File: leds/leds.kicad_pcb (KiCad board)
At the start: 4 copper layers, 68.8 x 135.2 mm, 96 parts, among them CN1 39302030, CN2 39288020, CN3 39288020, CN4 39288020, CN5 39302030, CN6 39288020, CN7 39288020, CN701 BM04B-SRSS-TB(LF)(SN), CN8 39288020, J202 Conn_01x06, J301 Conn_01x05_Pin, Q701 BSS138, Q702 BSS138, SW201 KEY-SMD_B3U-1000PM, SW202 KEY-SMD_B3U-1000PM, U1 SN74AHCT125PWR, U2 BTS70021EPPXUMA1, U201 ESP32-S3-WROOM-1, U3 BTS70021EPPXUMA1, U301 TPD6S300A, U302 TPS25730D, U401 TPS54202DDC, U402 CYA1040-15UH, U701 TPS73733DCQ_C5220270

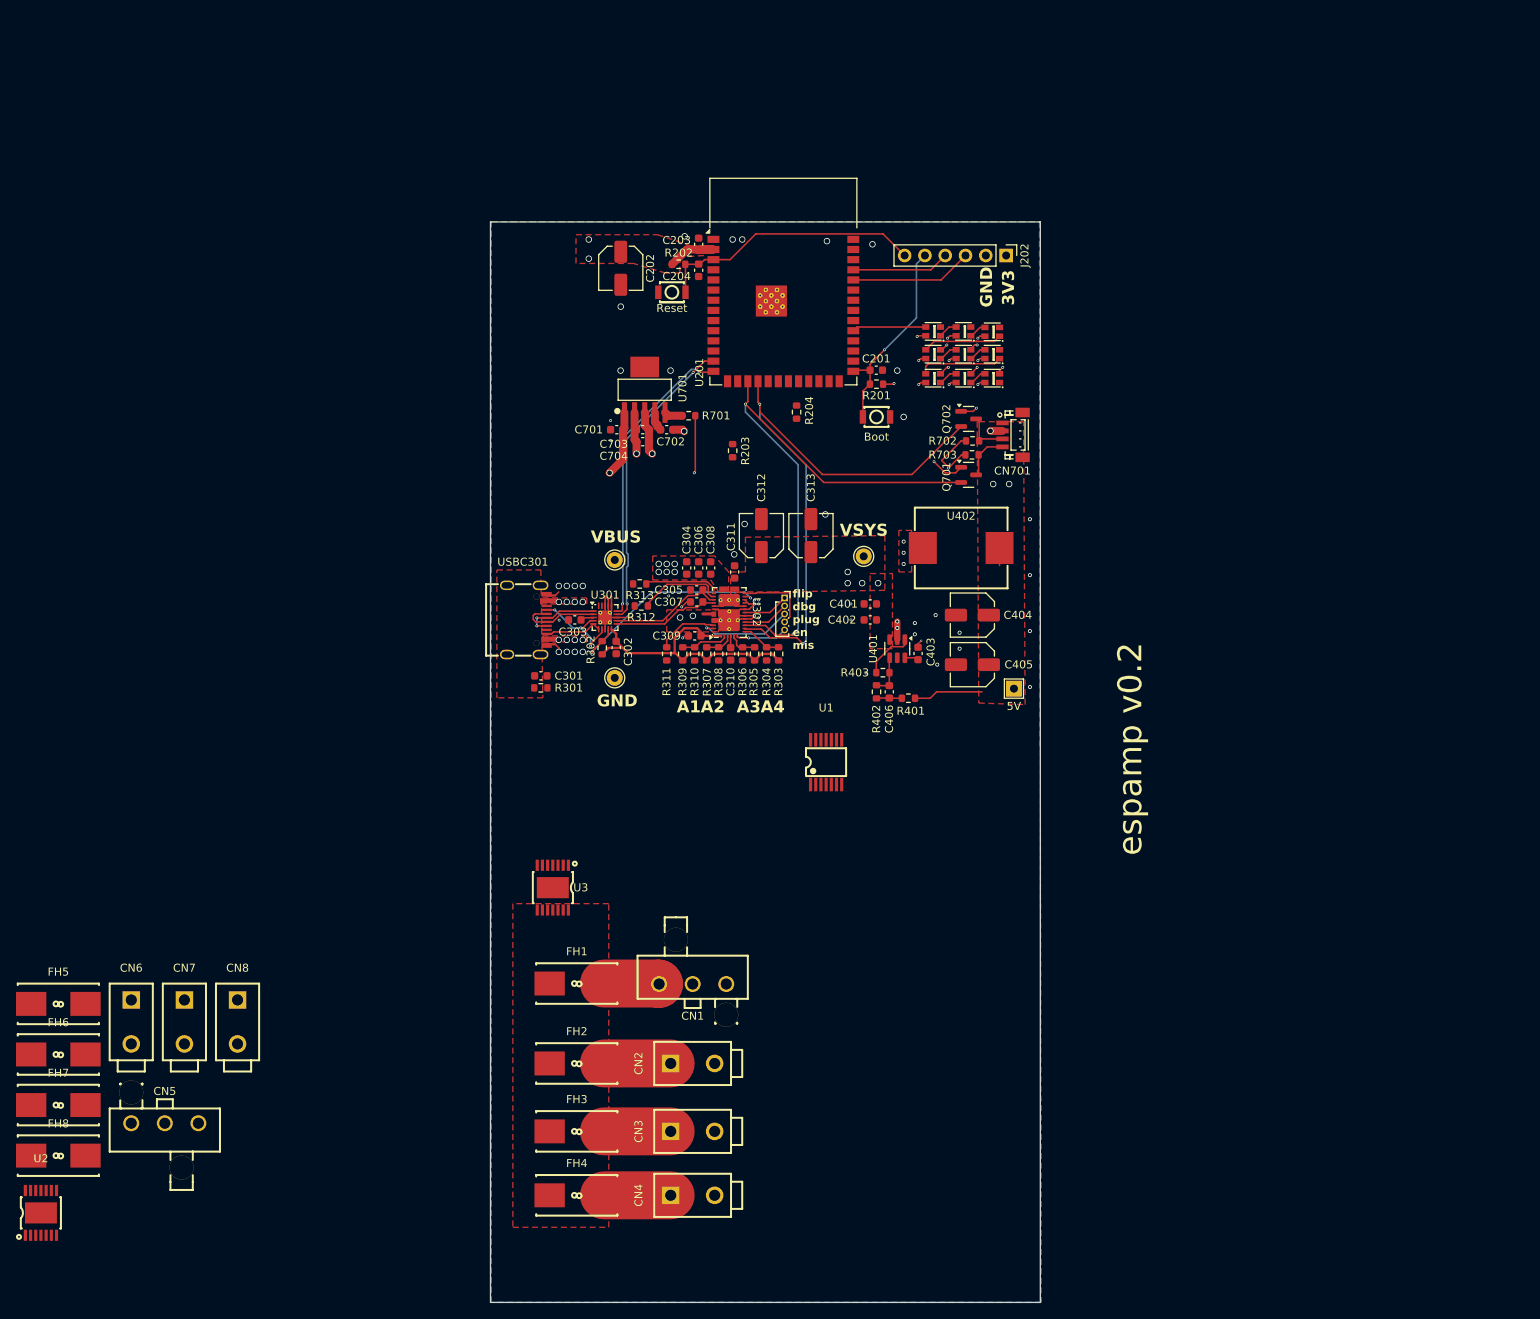
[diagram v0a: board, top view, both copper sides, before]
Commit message: first draft
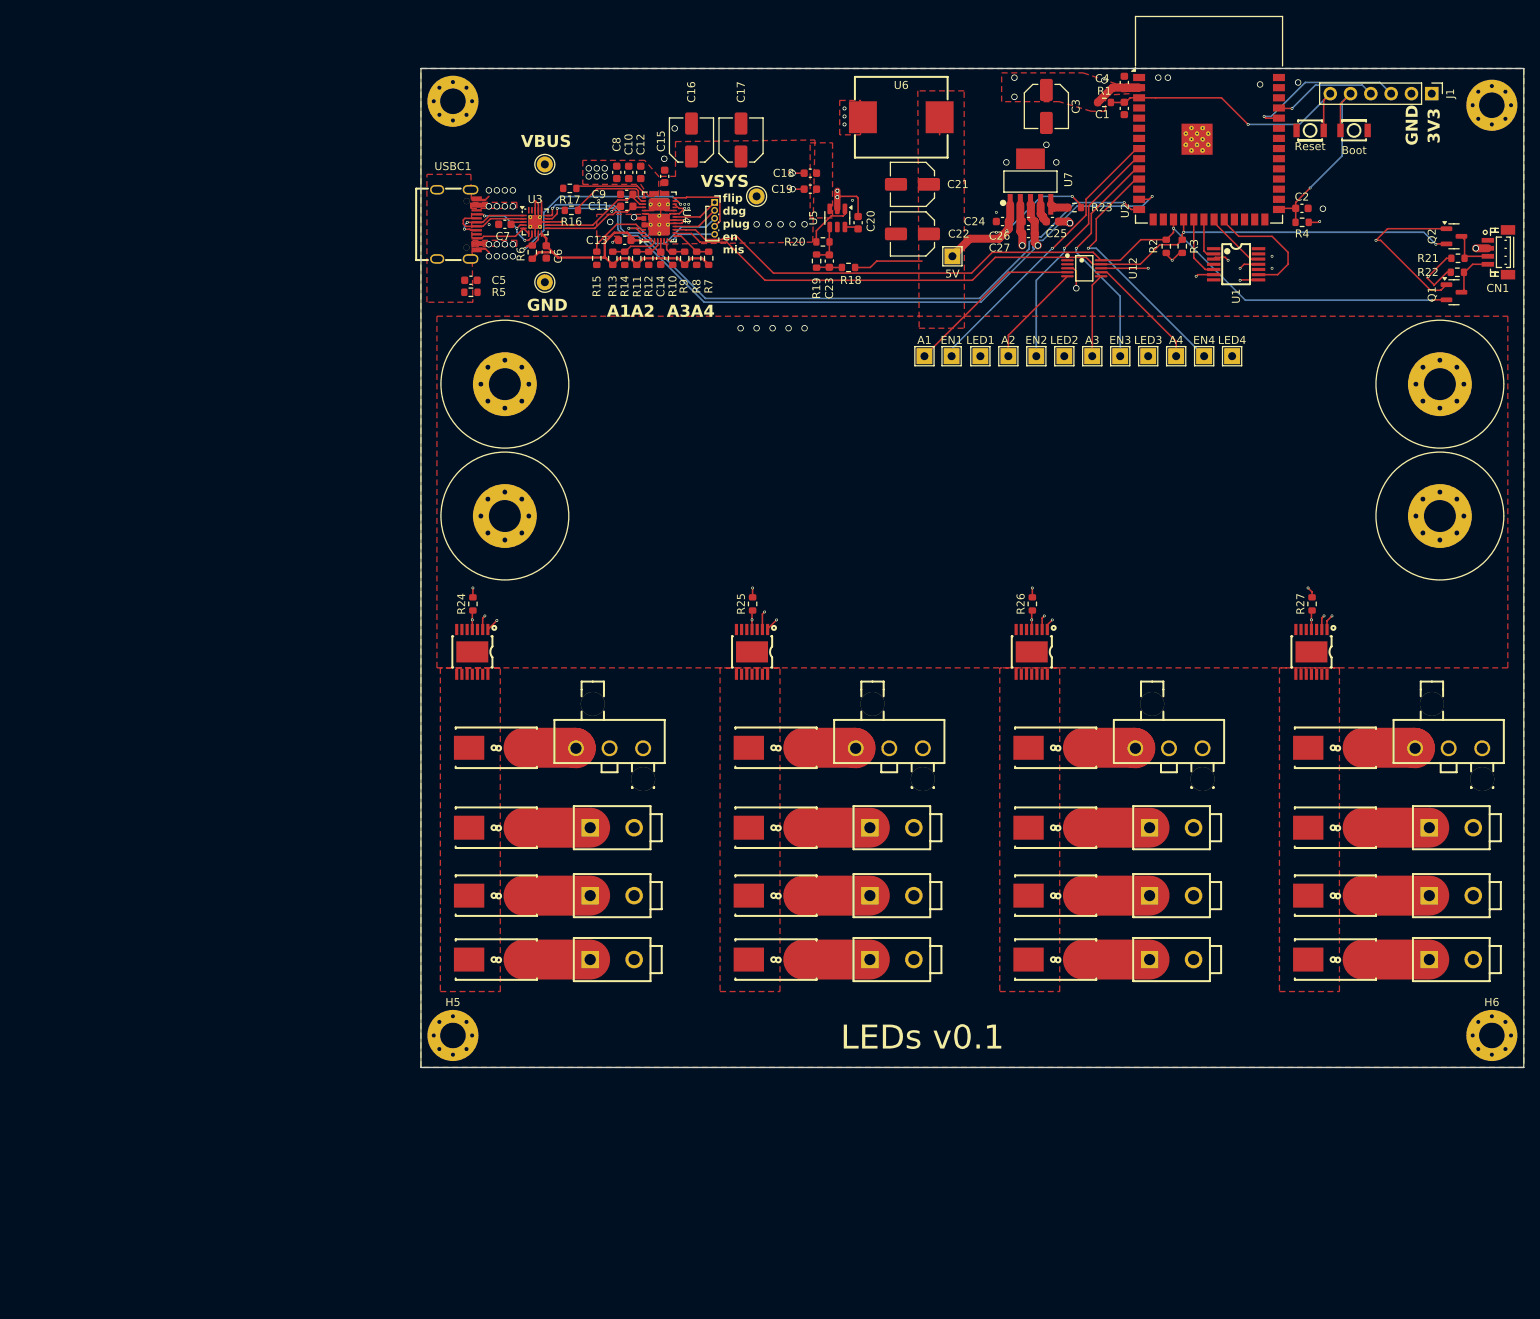
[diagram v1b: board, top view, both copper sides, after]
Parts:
- removed the CN5 at (-20.1, 157.0)
- removed LED201, LED202, LED203, LED204, LED205, LED206, LED207, LED208, LED209: WS2812B-2020, easyeda2kicad:LED-SMD_4P-L2.0-W2.0-TL_WS2812B-2020
- removed the U2 at (-35.5, 168.2)
- added CN10: 39302030, easyeda2kicad:CONN-TH_3P-P4.20_39302030, F.Cu at (105.6, 110.1)
- added CN11: 39288020, easyeda2kicad:CONN-TH_39288020, F.Cu at (105.9, 120.0)
- added CN12: 39288020, easyeda2kicad:CONN-TH_39288020, F.Cu at (105.9, 128.5)
- added CN13: 39288020, easyeda2kicad:CONN-TH_39288020, F.Cu at (105.9, 136.5)
- added CN14: 39302030, easyeda2kicad:CONN-TH_3P-P4.20_39302030, F.Cu at (140.6, 110.1)
- added CN15: 39288020, easyeda2kicad:CONN-TH_39288020, F.Cu at (140.9, 120.0)
- added CN16: 39288020, easyeda2kicad:CONN-TH_39288020, F.Cu at (140.9, 128.5)
- added CN17: 39288020, easyeda2kicad:CONN-TH_39288020, F.Cu at (140.9, 136.5)
- added CN9: 39288020, easyeda2kicad:CONN-TH_39288020, F.Cu at (70.9, 136.5)
- added FH10: 01550900M, easyeda2kicad:FUSE-SMD_L9.8-W5.0_01550900M, F.Cu at (91.4, 120.0)
- added FH11: 01550900M, easyeda2kicad:FUSE-SMD_L9.8-W5.0_01550900M, F.Cu at (91.4, 128.5)
- added FH12: 01550900M, easyeda2kicad:FUSE-SMD_L9.8-W5.0_01550900M, F.Cu at (91.4, 136.5)
- added FH13: 01550900M, easyeda2kicad:FUSE-SMD_L9.8-W5.0_01550900M, F.Cu at (126.4, 110.0)
- added FH14: 01550900M, easyeda2kicad:FUSE-SMD_L9.8-W5.0_01550900M, F.Cu at (126.4, 120.0)
- added FH15: 01550900M, easyeda2kicad:FUSE-SMD_L9.8-W5.0_01550900M, F.Cu at (126.4, 128.5)
- added FH16: 01550900M, easyeda2kicad:FUSE-SMD_L9.8-W5.0_01550900M, F.Cu at (126.4, 136.5)
- added FH9: 01550900M, easyeda2kicad:FUSE-SMD_L9.8-W5.0_01550900M, F.Cu at (91.4, 110.0)
- added H1: MountingHole_Pad, MountingHole:MountingHole_4mm_Pad_Via, F.Cu at (22.5, 81.0)
- added H2: MountingHole_Pad, MountingHole:MountingHole_4mm_Pad_Via, F.Cu at (139.5, 64.5)
- added H3: MountingHole_Pad, MountingHole:MountingHole_4mm_Pad_Via, F.Cu at (139.5, 81.0)
- added H4: MountingHole_Pad, MountingHole:MountingHole_4mm_Pad_Via, F.Cu at (22.5, 64.5)
- added H5: MountingHole_Pad, MountingHole:MountingHole_3.2mm_M3_Pad_Via, F.Cu at (16.0, 146.0)
- added H6: MountingHole_Pad, MountingHole:MountingHole_3.2mm_M3_Pad_Via, F.Cu at (146.0, 146.0)
- added H7: MountingHole_Pad, MountingHole:MountingHole_3.2mm_M3_Pad_Via, F.Cu at (16.0, 29.1)
- added H8: MountingHole_Pad, MountingHole:MountingHole_3.2mm_M3_Pad_Via, F.Cu at (146.0, 29.6)
- added R24: 820, Resistor_SMD:R_0603_1608Metric, F.Cu at (18.5, 92.0)
- added R25: 820, Resistor_SMD:R_0603_1608Metric, F.Cu at (53.5, 92.0)
- added R26: 820, Resistor_SMD:R_0603_1608Metric, F.Cu at (88.5, 92.0)
- added R27: 820, Resistor_SMD:R_0603_1608Metric, F.Cu at (123.5, 92.0)
- added TP10: LabeledTestPoint, easyeda2kicad:LabeledTestPoint, F.Cu at (89.0, 61.0)
- added TP11: LabeledTestPoint, easyeda2kicad:LabeledTestPoint, F.Cu at (99.5, 61.0)
- added TP12: LabeledTestPoint, easyeda2kicad:LabeledTestPoint, F.Cu at (110.0, 61.0)
- added TP13: LabeledTestPoint, easyeda2kicad:LabeledTestPoint, F.Cu at (75.0, 61.0)
- added TP14: LabeledTestPoint, easyeda2kicad:LabeledTestPoint, F.Cu at (85.5, 61.0)
- added TP15: LabeledTestPoint, easyeda2kicad:LabeledTestPoint, F.Cu at (96.0, 61.0)
- added TP16: LabeledTestPoint, easyeda2kicad:LabeledTestPoint, F.Cu at (106.5, 61.0)
- added TP5: LabeledTestPoint, easyeda2kicad:LabeledTestPoint, F.Cu at (82.0, 61.0)
- added TP6: LabeledTestPoint, easyeda2kicad:LabeledTestPoint, F.Cu at (92.5, 61.0)
- added TP7: LabeledTestPoint, easyeda2kicad:LabeledTestPoint, F.Cu at (103.0, 61.0)
- added TP8: LabeledTestPoint, easyeda2kicad:LabeledTestPoint, F.Cu at (113.5, 61.0)
- added TP9: LabeledTestPoint, easyeda2kicad:LabeledTestPoint, F.Cu at (78.4, 61.0)
- added U10: BTS70021EPPXUMA1, easyeda2kicad:PG-TSDSO-14_L4.9-W3.9-P0.65-LS6.0-BL-EP, F.Cu at (88.4, 98.0)
- added U11: BTS70021EPPXUMA1, easyeda2kicad:PG-TSDSO-14_L4.9-W3.9-P0.65-LS6.0-BL-EP, F.Cu at (123.4, 98.0)
- added U12: ADS1115IDGSR, easyeda2kicad:MSOP-10_L3.0-W3.0-P0.50-LS5.0-BL, F.Cu at (95.0, 50.0)
- added U9: BTS70021EPPXUMA1, easyeda2kicad:PG-TSDSO-14_L4.9-W3.9-P0.65-LS6.0-BL-EP, F.Cu at (53.4, 98.0)
- CN6: value 39288020 -> 39302030; footprint easyeda2kicad:CONN-TH_39288020 -> easyeda2kicad:CONN-TH_3P-P4.20_39302030
- moved CN6 100.8 mm to (70.6, 110.1), turned to 180 degrees
- moved FH5 95.3 mm to (56.4, 110.0)
- moved FH6 94.2 mm to (56.4, 120.0)
- moved FH7 93.5 mm to (56.4, 128.5)
- moved FH8 93.1 mm to (56.4, 136.5)
- moved CN7 91.8 mm to (70.9, 120.0), turned to 90 degrees
- moved CN8 83.4 mm to (70.9, 128.5), turned to 90 degrees
- moved SW1 82.4 mm to (123.3, 32.8)
- moved U1 80.7 mm to (114.0, 49.5), turned to -90 degrees
- moved SW2 69.7 mm to (128.8, 32.8)
- moved R22 64.9 mm to (141.7, 50.5)
- moved CN1 64.9 mm to (146.8, 48.0)
- moved Q1 64.9 mm to (141.3, 53.0)
- moved Q2 64.9 mm to (141.3, 46.0)
- moved R21 64.9 mm to (141.8, 48.8)
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- renumbered C204 to C1, C306 to C10, C307 to C11, C308 to C12, C309 to C13, C310 to C14, C311 to C15, C312 to C16, C313 to C17, C401 to C18, C402 to C19, C201 to C2, C403 to C20, C404 to C21, C405 to C22, C406 to C23, C701 to C24, C702 to C25, C703 to C26, C704 to C27, C202 to C3, C203 to C4, C301 to C5, C302 to C6, C303 to C7, C304 to C8, C305 to C9, CN701 to CN1, CN1 to CN2, CN2 to CN3, CN3 to CN4, CN4 to CN5, J202 to J1, J301 to J2, Q701 to Q1, Q702 to Q2, R202 to R1, R306 to R10, R307 to R11, R308 to R12, R309 to R13, R310 to R14, R311 to R15, R312 to R16, R313 to R17, R401 to R18, R402 to R19, R203 to R2, R403 to R20, R702 to R21, R703 to R22, R701 to R23, R204 to R3, R201 to R4, R301 to R5, R302 to R6, R303 to R7, R304 to R8, R305 to R9, SW202 to SW1, SW201 to SW2, TP301 to TP1, TP302 to TP2, TP303 to TP3, TP401 to TP4, U201 to U2, U301 to U3, U302 to U4, U401 to U5, U402 to U6, U701 to U7, U3 to U8, USBC301 to USBC1
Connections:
- net /esp32/I2C.SCL renamed /a2d/I2C.SCL
- net /esp32/I2C.SDA renamed /a2d/I2C.SDA
- CN2 pad 1: (no net) -> Net-(CN2-Pad1)
- CN2 pad 2: /led_channel/DIN -> /esp32/LED1
- CN3 pad 1: unconnected-(FH2-Pad2) -> Net-(CN3-Pad1)
- CN6 pad 2: GND -> /esp32/LED2
- FH1 pad 2: (no net) -> Net-(CN2-Pad1)
- FH2 pad 2: unconnected-(FH2-Pad2) -> Net-(CN3-Pad1)
- FH5 pad 2: Net-(CN5-Pad1) (its old number) -> Net-(CN6-Pad1)
- FH6 pad 2: Net-(CN6-Pad1) -> Net-(CN7-Pad1)
- FH7 pad 2: Net-(CN7-Pad1) -> Net-(CN8-Pad1)
- FH8 pad 2: Net-(CN8-Pad1) -> Net-(CN9-Pad1)
- U1 pad 1: unconnected-(U1-~{1OE}-Pad1) -> GND
- U1 pad 10: unconnected-(U1-~{3OE}-Pad10) -> GND
- U1 pad 11: unconnected-(U1-4Y-Pad11) -> /esp32/LED3
- U1 pad 12: unconnected-(U1-4A-Pad12) -> Net-(U1-4A)
- U1 pad 13: unconnected-(U1-~{4OE}-Pad13) -> GND
- U1 pad 2: unconnected-(U1-1A-Pad2) -> Net-(U1-1A)
- U1 pad 3: unconnected-(U1-1Y-Pad3) -> /esp32/LED2
- U1 pad 4: unconnected-(U1-~{2OE}-Pad4) -> GND
- U1 pad 5: unconnected-(U1-2A-Pad5) -> Net-(U1-2A)
- U1 pad 6: unconnected-(U1-2Y-Pad6) -> /esp32/LED1
- U1 pad 7: unconnected-(U1-GND-Pad7) -> GND
- U1 pad 8: unconnected-(U1-3Y-Pad8) -> /esp32/LED4
- U1 pad 9: unconnected-(U1-3A-Pad9) -> Net-(U1-3A)
- U2 pad 10: unconnected-(U201-IO17-Pad10) -> /esp32/EN3
- U2 pad 11: unconnected-(U201-IO18-Pad11) -> /esp32/EN4
- U2 pad 19: unconnected-(U201-IO11-Pad19) -> Net-(U1-2A)
- U2 pad 20: unconnected-(U201-IO12-Pad20) -> Net-(U1-1A)
- U2 pad 21: unconnected-(U201-IO13-Pad21) -> Net-(U1-4A)
- U2 pad 22: unconnected-(U201-IO14-Pad22) -> Net-(U1-3A)
- U2 pad 31: Net-(LED201-DI) -> unconnected-(U2-IO38-Pad31)
- U2 pad 8: unconnected-(U201-IO15-Pad8) -> /esp32/EN1
- U2 pad 9: unconnected-(U201-IO16-Pad9) -> /esp32/EN2
- U8 pad 11: (no net) -> unconnected-(U8-n.c.-Pad11)
- U8 pad 15: /led_channel/12V -> /buckconverter/VIN
- U8 pad 2: /led_channel/IN -> /esp32/EN1
- U8 pad 4: /led_channel/IS -> /a2d/AIN1
- U8 pad 5: (no net) -> unconnected-(U8-n.c.-Pad5)
- U8 pad 6: (no net) -> unconnected-(U8-n.c.-Pad6)
- U8 pad 7: (no net) -> unconnected-(U8-n.c.-Pad7)
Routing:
- net /esp32/LED1: track 0.00 -> 112.0 mm, vias 0 -> 1
- net /esp32/EN1: track 0.00 -> 109.6 mm, vias 0 -> 2
- net /a2d/AIN1: track 0.00 -> 94.9 mm, vias 0 -> 1
- net /esp32/LED2: track 0.00 -> 88.6 mm, vias 0 -> 1
- net /esp32/EN2: track 0.00 -> 79.8 mm, vias 0 -> 2
- net /esp32/LED4: track 0.00 -> 72.5 mm, vias 0 -> 1
- net /esp32/EN4: track 0.00 -> 72.1 mm, vias 0 -> 2
- net /5V: track 51.8 -> 123.2 mm, vias 15 -> 5
- net /esp32/LED3: track 0.00 -> 68.7 mm, vias 0 -> 1
- net /esp32/EN3: track 0.00 -> 67.4 mm, vias 0 -> 2
- net /a2d/AIN2: track 0.00 -> 61.8 mm, vias 0 -> 1
- net /a2d/AIN4: track 0.00 -> 57.2 mm, vias 0 -> 1
- net /esp32/USB.DN: track 38.0 -> 90.7 mm
- net /esp32/USB.DP: track 37.4 -> 87.0 mm
- net /a2d/AIN3: track 0.00 -> 49.0 mm, vias 0 -> 1
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- added copper zone on F.Cu, net /led_channel/Switched12V
- added copper zone on F.Cu, net /led_channel1/Switched12V
- added copper zone on F.Cu, net /led_channel2/Switched12V
- added copper zone on F.Cu, net /led_channel3/Switched12V
- added copper zone on F.Cu, net GND
- added copper zone on In2.Cu, net GND
- removed copper zone on F.Cu, net /led_channel/12V
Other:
- board size 68.8 x 135.2 mm -> 138 x 125 mm
- board text added: "LEDs v0.1"
- board text removed: "espamp v0.2"
